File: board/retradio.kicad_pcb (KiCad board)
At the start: 2 copper layers, 39 x 56 mm, 26 parts, among them J1 Power, J2 Speaker, M1 Orange-Pi-Zero, U1 NCP1117-5.0_SOT223, U2 PAM8320, X1 I2C-6P

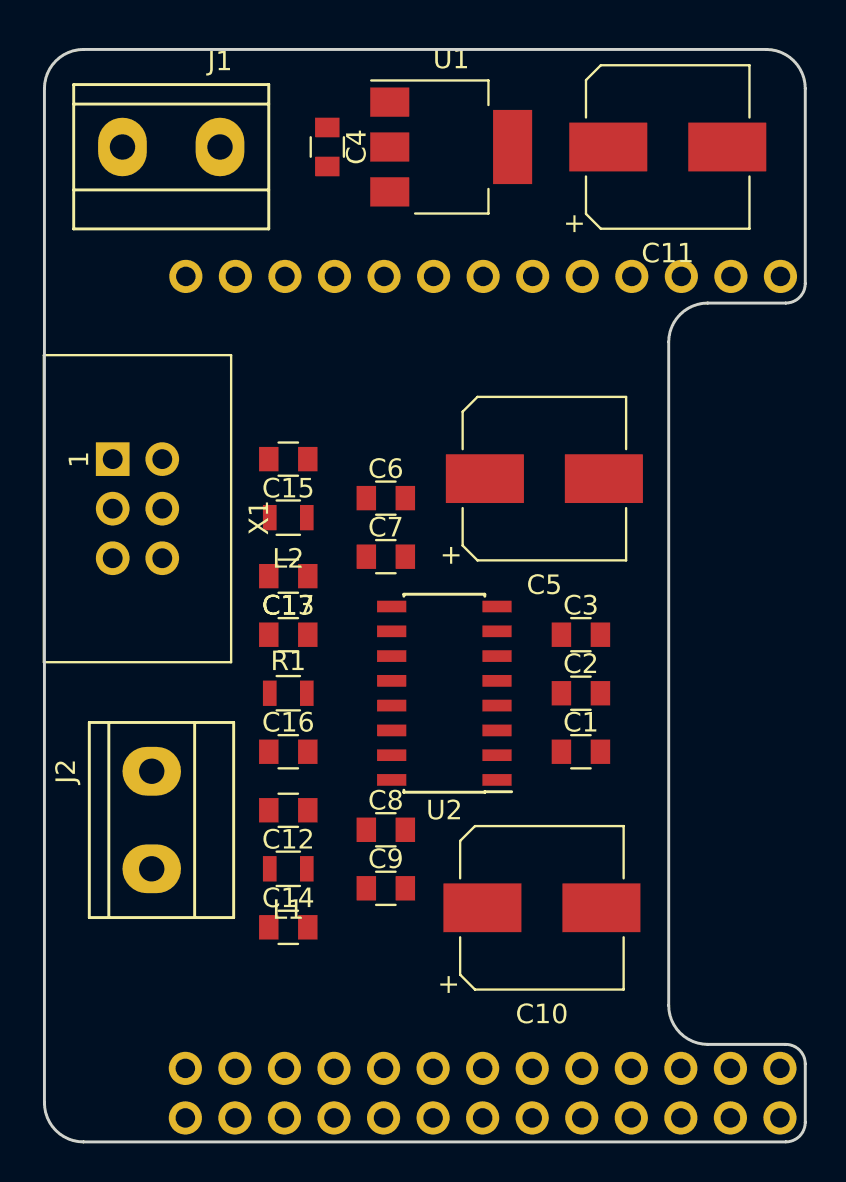
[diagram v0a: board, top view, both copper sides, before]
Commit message: WIP
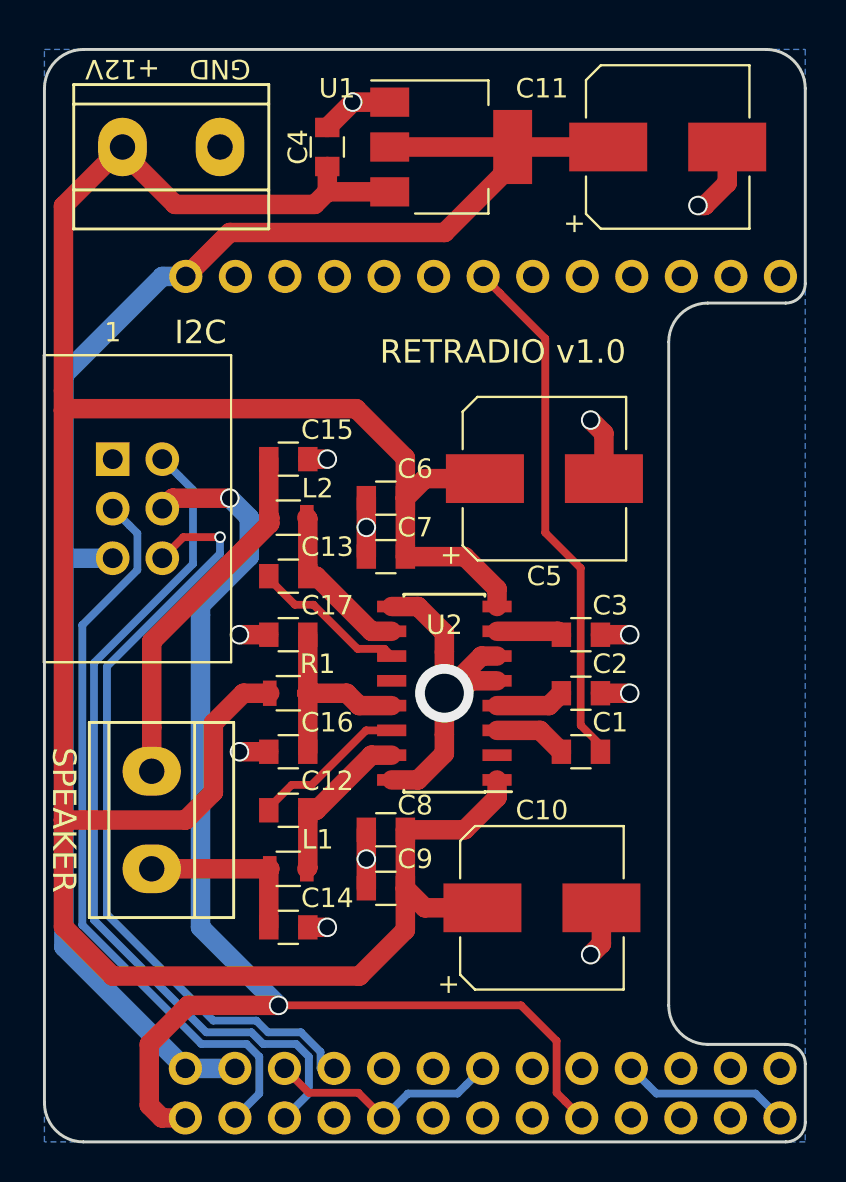
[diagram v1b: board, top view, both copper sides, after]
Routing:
- net +12V: track 0.00 -> 143.7 mm
- net +5V: track 0.00 -> 82.8 mm
- net GND: track 0.00 -> 67.6 mm, vias 0 -> 13
- net +3V3: track 0.00 -> 65.0 mm, vias 0 -> 2
- net /SCL: track 0.00 -> 44.0 mm
- net /ALERT: track 0.00 -> 40.5 mm, vias 0 -> 1
- net /SDA: track 0.00 -> 38.6 mm
- net /AUDIO: track 0.00 -> 26.9 mm
- net Net-(C15-Pad2): track 0.00 -> 18.5 mm
- net /AVCC: track 0.00 -> 10.7 mm
- net Net-(C14-Pad1): track 0.00 -> 9.07 mm
- net Net-(C13-Pad1): track 0.00 -> 8.56 mm
- net Net-(C12-Pad1): track 0.00 -> 8.56 mm
- net Net-(C13-Pad2): track 0.00 -> 8.07 mm
- net Net-(C12-Pad2): track 0.00 -> 8.07 mm
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- added copper zone on B.Cu, net GND
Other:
- net class Default: trace_width 0.25 -> 0.4
- net class PWR added: clearance 0.2, trace_width 1, via_dia 1, via_drill 0.8
- board text added: "+12V"
- board text added: "GND"
- board text added: "I2C"
- board text added: "RETRADIO v1.0"
- board text added: "SPEAKER"
